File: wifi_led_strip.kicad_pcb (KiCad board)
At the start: 2 copper layers, 14 parts, among them J1 Serial, J2 Power, J3 ESP01, J4 Leds, SW1 Flash, SW2 Reset, U1 TLV1117-33

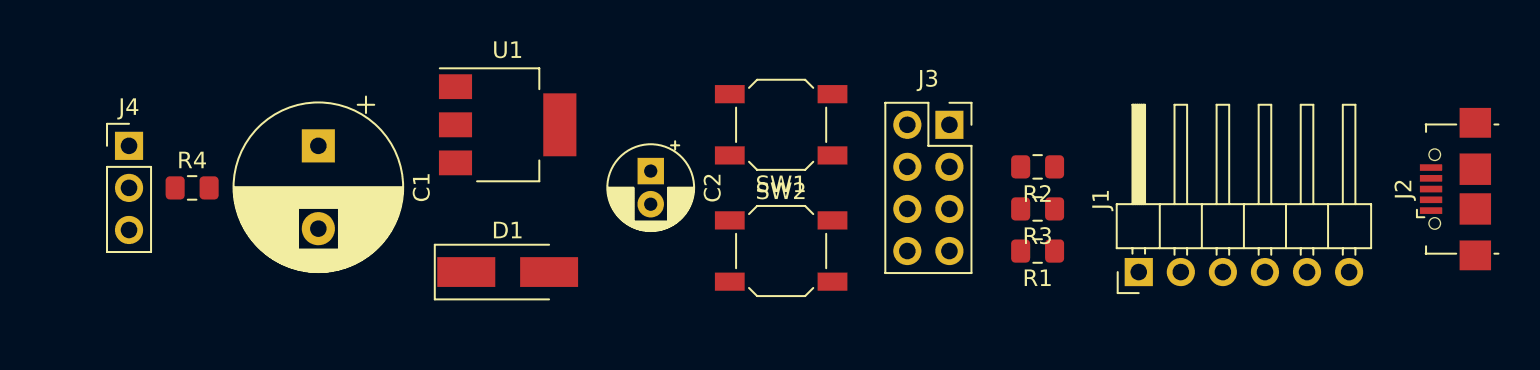
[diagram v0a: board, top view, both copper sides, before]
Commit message: place components and labels
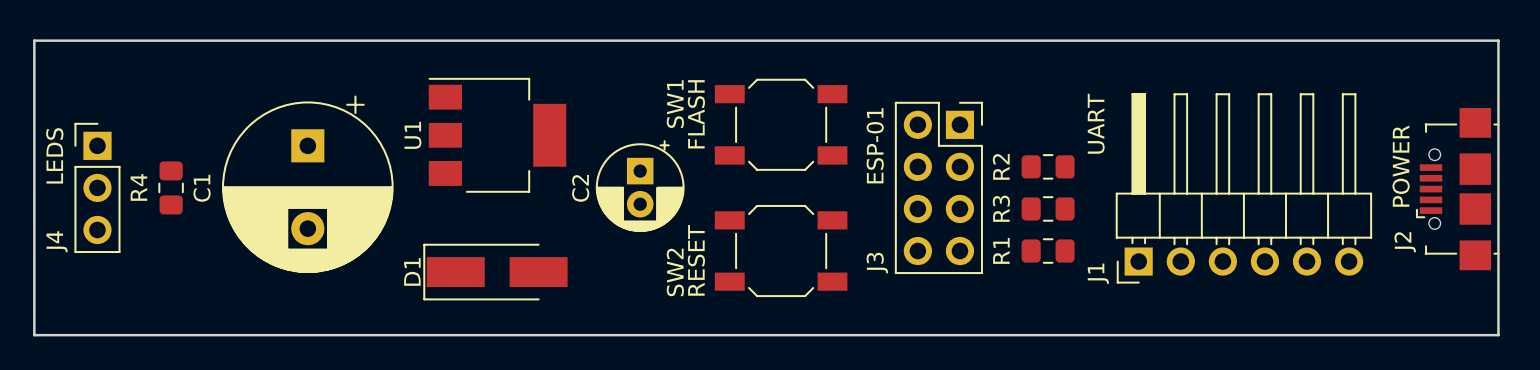
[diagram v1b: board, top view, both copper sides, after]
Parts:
- moved J4 1.91 mm to (117.5, 104.1)
- moved R4 1.27 mm to (121.9, 106.7), turned to 270 degrees
- moved U1 0.88 mm to (141.6, 103.5)
- moved D1 0.64 mm to (141.6, 111.8)
- moved J1 0.64 mm to (180.3, 111.1)
- moved C1 0.63 mm to (130.2, 104.1)
- moved C2 0.63 mm to (150.2, 105.7)
- moved J3 0.63 mm to (169.5, 102.9)
- moved R1 0.63 mm to (174.9, 110.5)
- moved R2 0.63 mm to (174.9, 105.4)
- moved R3 0.63 mm to (174.9, 108.0)
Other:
- board outline added: 88.4 x 17.8 mm
- board text added: "ESP-01"
- board text added: "FLASH"
- board text added: "LEDS"
- board text added: "POWER"
- board text added: "RESET"
- board text added: "UART"
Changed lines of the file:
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@@
   (general
     (thickness 1.6)
-    (drawings 1)
+    (drawings 10)
     (tracks 0)
     (zones 0)
@@
     (46 B.CrtYd user)
     (47 F.CrtYd user)
-    (48 B.Fab user)
-    (49 F.Fab user)
+    (48 B.Fab user hide)
+    (49 F.Fab user hide)
   )
   (setup
@@
   )
   (module Capacitor_THT:CP_Radial_D10.0mm_P5.00mm (layer F.Cu)
-    (at 130.81 104.14 270)
+    (at 130.175 104.14 270)
     (descr "CP, Radial series, Radial, pin pitch=5.00mm, , diameter=10mm, Electrolytic Capacitor")
     (tags "CP Radial series Radial pin pitch 5.00mm  diameter 10mm Electrolytic Capacitor")
-    (fp_text reference C1 (at 2.5 -6.25 270) (layer F.SilkS)
+    (fp_text reference C1 (at 2.54 6.35 270) (layer F.SilkS)
       (effects (font (size 1 1) (thickness 0.15)))
     )
@@
   )
   (module Capacitor_THT:CP_Radial_D5.0mm_P2.00mm (layer F.Cu)
-    (at 150.876 105.664 270)
+    (at 150.241 105.664 270)
     (descr "CP, Radial series, Radial, pin pitch=2.00mm, , diameter=5mm, Electrolytic Capacitor")
     (tags "CP Radial series Radial pin pitch 2.00mm  diameter 5mm Electrolytic Capacitor")
-    (fp_text reference C2 (at 1 -3.75 270) (layer F.SilkS)
+    (fp_text reference C2 (at 1.016 3.556 270) (layer F.SilkS)
       (effects (font (size 1 1) (thickness 0.15)))
     )
@@
   )
   (module Diode_SMD:D_SMA_Handsoldering (layer F.Cu)
-    (at 142.24 111.76)
+    (at 141.605 111.76)
     (descr "Diode SMA (DO-214AC) Handsoldering")
     (tags "Diode SMA (DO-214AC) Handsoldering")
     (attr smd)
-    (fp_text reference D1 (at 0 -2.5) (layer F.SilkS)
+    (fp_text reference D1 (at -5.08 0 90) (layer F.SilkS)
       (effects (font (size 1 1) (thickness 0.15)))
     )
@@
   )
   (module Connector_PinHeader_2.54mm:PinHeader_1x06_P2.54mm_Horizontal (layer F.Cu)
-    (at 180.34 111.76 90)
+    (at 180.34 111.125 90)
     (descr "Through hole angled pin header, 1x06, 2.54mm pitch, 6mm pin length, single row")
     (tags "Through hole angled pin header THT 1x06 2.54mm single row")
-    (fp_text reference J1 (at 4.385 -2.27 90) (layer F.SilkS)
+    (fp_text reference J1 (at -0.635 -2.54 90) (layer F.SilkS)
       (effects (font (size 1 1) (thickness 0.15)))
     )
@@
     (tags "Micro-USB SMD Typ-B")
     (attr smd)
-    (fp_text reference J2 (at 0 -4.325 90) (layer F.SilkS)
+    (fp_text reference J2 (at -3.105 -4.325 90) (layer F.SilkS)
       (effects (font (size 1 1) (thickness 0.15)))
     )
@@
   )
   (module Connector_PinSocket_2.54mm:PinSocket_2x04_P2.54mm_Vertical (layer F.Cu)
-    (at 168.91 102.87)
+    (at 169.545 102.87)
     (descr "Through hole straight socket strip, 2x04, 2.54mm pitch, double cols (from Kicad 4.0.7), script generated")
     (tags "Through hole socket strip THT 2x04 2.54mm double row")
-    (fp_text reference J3 (at -1.27 -2.77) (layer F.SilkS)
+    (fp_text reference J3 (at -5.08 8.255 90) (layer F.SilkS)
       (effects (font (size 1 1) (thickness 0.15)))
     )
@@
   )
   (module Connector_PinHeader_2.54mm:PinHeader_1x03_P2.54mm_Vertical (layer F.Cu)
-    (at 119.38 104.14)
+    (at 117.475 104.14)
     (descr "Through hole straight pin header, 1x03, 2.54mm pitch, single row")
     (tags "Through hole pin header THT 1x03 2.54mm single row")
-    (fp_text reference J4 (at 0 -2.33) (layer F.SilkS)
+    (fp_text reference J4 (at -2.54 5.715 90) (layer F.SilkS)
       (effects (font (size 1 1) (thickness 0.15)))
     )
@@
   )
   (module Resistor_SMD:R_0805_2012Metric_Pad1.15x1.40mm_HandSolder (layer F.Cu)
-    (at 174.235 110.49 180)
+    (at 174.87 110.49 180)
     (descr "Resistor SMD 0805 (2012 Metric), square (rectangular) end terminal, IPC_7351 nominal with elongated pad for handsoldering. (Body size source: https://docs.google.com/spreadsheets/d/1BsfQQcO9C6DZCsRaXUlFlo91Tg2WpOkGARC1WS5S8t0/edit?usp=sharing), generated with kicad-footprint-generator")
     (tags "resistor handsolder")
     (attr smd)
-    (fp_text reference R1 (at 0 -1.65 180) (layer F.SilkS)
+    (fp_text reference R1 (at 2.785 0 270) (layer F.SilkS)
       (effects (font (size 1 1) (thickness 0.15)))
     )
@@
   )
   (module Resistor_SMD:R_0805_2012Metric_Pad1.15x1.40mm_HandSolder (layer F.Cu)
-    (at 174.235 105.41 180)
+    (at 174.87 105.41 180)
     (descr "Resistor SMD 0805 (2012 Metric), square (rectangular) end terminal, IPC_7351 nominal with elongated pad for handsoldering. (Body size source: https://docs.google.com/spreadsheets/d/1BsfQQcO9C6DZCsRaXUlFlo91Tg2WpOkGARC1WS5S8t0/edit?usp=sharing), generated with kicad-footprint-generator")
     (tags "resistor handsolder")
     (attr smd)
-    (fp_text reference R2 (at 0 -1.65 180) (layer F.SilkS)
+    (fp_text reference R2 (at 2.785 0 270) (layer F.SilkS)
       (effects (font (size 1 1) (thickness 0.15)))
     )
@@
   )
   (module Resistor_SMD:R_0805_2012Metric_Pad1.15x1.40mm_HandSolder (layer F.Cu)
-    (at 174.235 107.95 180)
+    (at 174.87 107.95 180)
     (descr "Resistor SMD 0805 (2012 Metric), square (rectangular) end terminal, IPC_7351 nominal with elongated pad for handsoldering. (Body size source: https://docs.google.com/spreadsheets/d/1BsfQQcO9C6DZCsRaXUlFlo91Tg2WpOkGARC1WS5S8t0/edit?usp=sharing), generated with kicad-footprint-generator")
     (tags "resistor handsolder")
     (attr smd)
-    (fp_text reference R3 (at 0 -1.65 180) (layer F.SilkS)
+    (fp_text reference R3 (at 2.785 0 270) (layer F.SilkS)
       (effects (font (size 1 1) (thickness 0.15)))
     )
@@
   )
   (module Resistor_SMD:R_0805_2012Metric_Pad1.15x1.40mm_HandSolder (layer F.Cu)
-    (at 123.19 106.68)
+    (at 121.92 106.68 270)
     (descr "Resistor SMD 0805 (2012 Metric), square (rectangular) end terminal, IPC_7351 nominal with elongated pad for handsoldering. (Body size source: https://docs.google.com/spreadsheets/d/1BsfQQcO9C6DZCsRaXUlFlo91Tg2WpOkGARC1WS5S8t0/edit?usp=sharing), generated with kicad-footprint-generator")
     (tags "resistor handsolder")
     (attr smd)
-    (fp_text reference R4 (at 0 -1.65) (layer F.SilkS)
-      (effects (font (size 1 1) (thickness 0.15)))
-    )
-    (fp_text value 470 (at 0 1.65) (layer F.Fab)
-      (effects (font (size 1 1) (thickness 0.15)))
-    )
-    (fp_text user %R (at 0 0) (layer F.Fab)
+    (fp_text reference R4 (at 0 1.905 90) (layer F.SilkS)
+      (effects (font (size 1 1) (thickness 0.15)))
+    )
+    (fp_text value 470 (at 0 1.65 270) (layer F.Fab)
+      (effects (font (size 1 1) (thickness 0.15)))
+    )
+    (fp_text user %R (at 0 0 270) (layer F.Fab)
       (effects (font (size 0.5 0.5) (thickness 0.08)))
     )
@@
     (fp_line (start -1 -0.6) (end 1 -0.6) (layer F.Fab) (width 0.1))
     (fp_line (start -1 0.6) (end -1 -0.6) (layer F.Fab) (width 0.1))
-    (pad 2 smd roundrect (at 1.025 0) (size 1.15 1.4) (layers F.Cu F.Paste F.Mask) (roundrect_rratio 0.217391)
+    (pad 2 smd roundrect (at 1.025 0 270) (size 1.15 1.4) (layers F.Cu F.Paste F.Mask) (roundrect_rratio 0.217391)
       (net 11 /GPIO2))
-    (pad 1 smd roundrect (at -1.025 0) (size 1.15 1.4) (layers F.Cu F.Paste F.Mask) (roundrect_rratio 0.217391)
+    (pad 1 smd roundrect (at -1.025 0 270) (size 1.15 1.4) (layers F.Cu F.Paste F.Mask) (roundrect_rratio 0.217391)
       (net 15 "Net-(J4-Pad2)"))
     (model ${KISYS3DMOD}/Resistor_SMD.3dshapes/R_0805_2012Metric.wrl
@@
     (tags "SPST Button Switch")
     (attr smd)
-    (fp_text reference SW1 (at 0 -3.6 180) (layer F.SilkS)
+    (fp_text reference SW1 (at 6.35 1.27 270) (layer F.SilkS)
       (effects (font (size 1 1) (thickness 0.15)))
     )
@@
     (tags "SPST Button Switch")
     (attr smd)
-    (fp_text reference SW2 (at 0 -3.6) (layer F.SilkS)
+    (fp_text reference SW2 (at -6.35 1.27 90) (layer F.SilkS)
       (effects (font (size 1 1) (thickness 0.15)))
     )
@@
   )
   (module Package_TO_SOT_SMD:SOT-223-3_TabPin2 (layer F.Cu)
-    (at 142.24 102.87)
+    (at 141.63 103.505)
     (descr "module CMS SOT223 4 pins")
     (tags "CMS SOT")
     (attr smd)
-    (fp_text reference U1 (at 0 -4.5) (layer F.SilkS)
+    (fp_text reference U1 (at -5.08 0 90) (layer F.SilkS)
       (effects (font (size 1 1) (thickness 0.15)))
     )
@@
     )
   )
-  (gr_line (start 207.01 106.68) (end 115.57 106.68) (layer Dwgs.User) (width 0.2))
+  (gr_text LEDS (at 114.935 104.775 90) (layer F.SilkS)
+    (effects (font (size 1 1) (thickness 0.15)))
+  )
+  (gr_text RESET (at 153.67 111.125 90) (layer F.SilkS)
+    (effects (font (size 1 1) (thickness 0.15)))
+  )
+  (gr_text FLASH (at 153.67 102.235 90) (layer F.SilkS)
+    (effects (font (size 1 1) (thickness 0.15)))
+  )
+  (gr_text ESP-01 (at 164.465 104.14 90) (layer F.SilkS)
+    (effects (font (size 1 1) (thickness 0.15)))
+  )
+  (gr_text POWER (at 196.215 105.41 90) (layer F.SilkS)
+    (effects (font (size 1 1) (thickness 0.15)))
+  )
+  (gr_text UART (at 177.8 102.87 90) (layer F.SilkS)
+    (effects (font (size 1 1) (thickness 0.15)))
+  )
+  (gr_line (start 202.057 115.57) (end 113.665 115.57) (layer Edge.Cuts) (width 0.15))
+  (gr_line (start 202.057 97.79) (end 202.057 115.57) (layer Edge.Cuts) (width 0.15))
+  (gr_line (start 113.665 97.79) (end 202.057 97.79) (layer Edge.Cuts) (width 0.15))
+  (gr_line (start 113.665 115.57) (end 113.665 97.79) (layer Edge.Cuts) (width 0.15))
 )

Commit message: finish routing
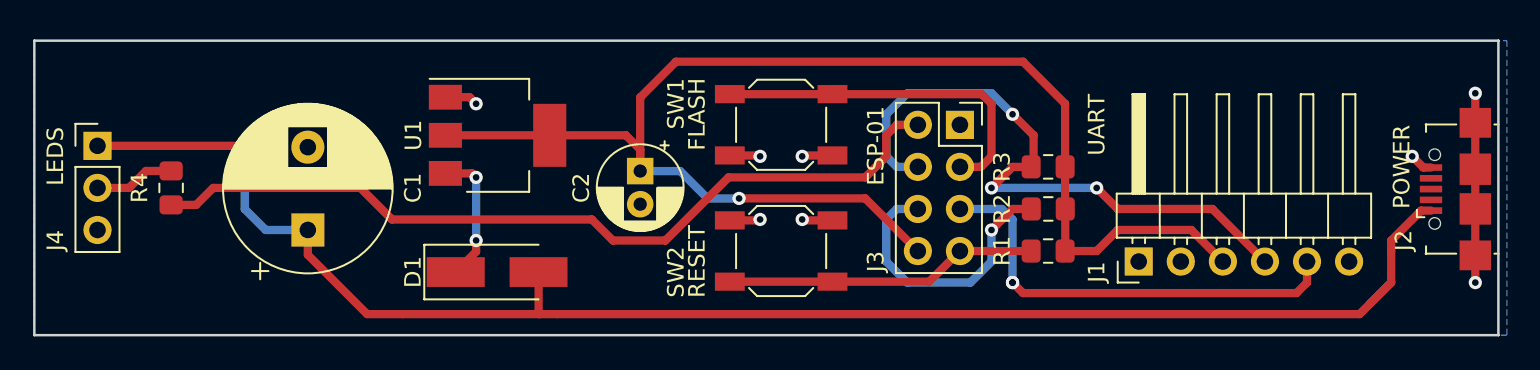
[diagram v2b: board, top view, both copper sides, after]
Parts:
- moved C1 5.08 mm to (130.2, 109.2), turned to 90 degrees
- moved R2 2.54 mm to (174.9, 108.0)
- moved R3 2.54 mm to (174.9, 105.4)
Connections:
- net /CH_PD renamed Net-(J3-Pad6)
- net /CTSn renamed Net-(J1-Pad2)
- net /GPIO0 renamed /FLASH
- net /GPIO2 renamed Net-(J3-Pad2)
- net /RTSn renamed Net-(J1-Pad6)
- J1 pad 4: /RXD -> /PC_TO_ESP
- J1 pad 5: /RXD -> /ESP_TO_PC
- J3 pad 4: /RXD -> /PC_TO_ESP
- J3 pad 5: /RXD -> /ESP_TO_PC
- R3 pad 2: /RXD -> /PC_TO_ESP
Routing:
- net /5V: track 0.00 -> 96.3 mm, vias 0 -> 1
- net /3V3: track 0.00 -> 84.0 mm, vias 0 -> 1
- net Net-(J3-Pad2): track 0.00 -> 50.5 mm
- net /PC_TO_ESP: track 0.00 -> 38.4 mm, vias 0 -> 3
- net /ESP_TO_PC: track 0.00 -> 26.8 mm, vias 0 -> 2
- net /GND: track 0.00 -> 22.3 mm, vias 0 -> 8
- net /FLASH: track 0.00 -> 21.4 mm
- net /RESET: track 0.00 -> 19.0 mm
- net Net-(J3-Pad6): track 0.00 -> 16.9 mm, vias 0 -> 1
- net Net-(D1-Pad1): track 0.00 -> 8.18 mm, vias 0 -> 2
- net Net-(J4-Pad2): track 0.00 -> 4.87 mm
- added copper zone on B.Cu, net /GND
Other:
- net class Default: trace_width 0.25 -> 0.5
- net class Small Signals added: clearance 0.2, trace_width 0.25, via_dia 0.8, via_drill 0.4
